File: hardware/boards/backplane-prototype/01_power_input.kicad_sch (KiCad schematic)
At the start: 13 parts, among them J5 DC IN, U4 INA237AIDGSR

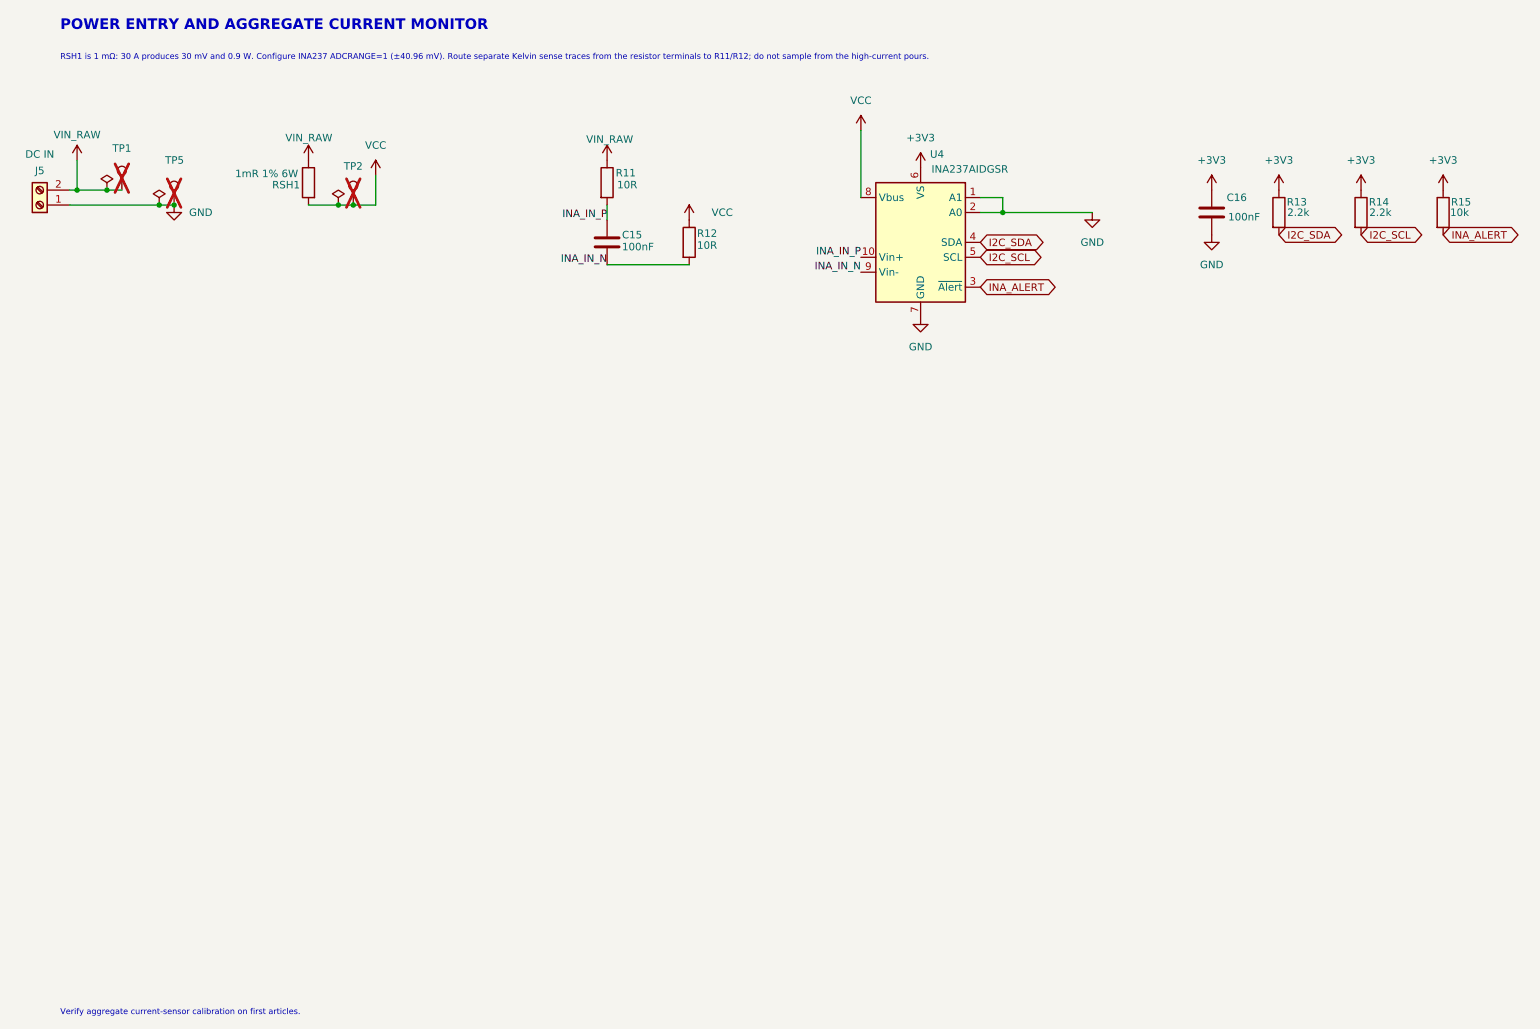
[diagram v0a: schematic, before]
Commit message: checkpoint: save schematic updates
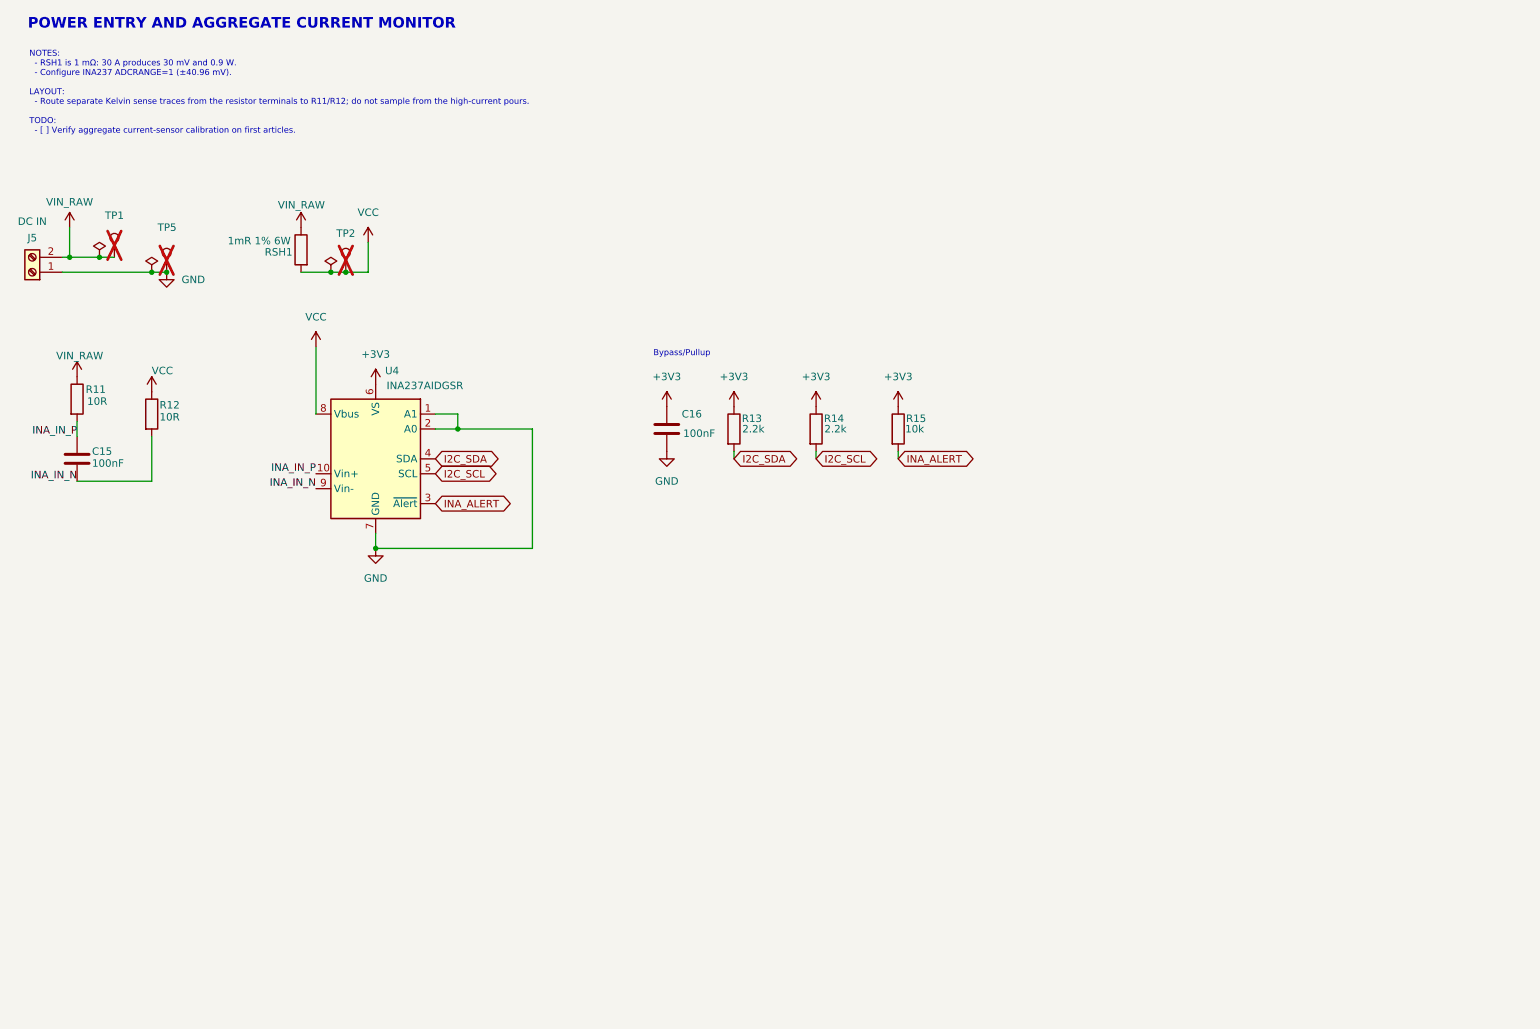
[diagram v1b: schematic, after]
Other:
- note added: "Bypass/Pullup"
- note added: "NOTES: - RSH1 is 1 mΩ: 30 A produces 30 mV and 0.9 W. - Configure INA237 ADCRANGE=1 (±40.96 mV). LAYOUT: - Route separate Kelvin sense traces from the resistor terminals to R11/R12; do not sample from the high-current pours. TODO:r - [ ] Verify aggregate current-sensor calibration on first articles."
- note removed: "RSH1 is 1 mΩ: 30 A produces 30 mV and 0.9 W. Configure INA237 ADCRANGE=1 (±40.96 mV). Route separate Kelvin sense traces from the resistor terminals to R11/R12; do not sample from the high-current pours."
- note removed: "Verify aggregate current-sensor calibration on first articles."
- moved on the sheet: C15, C16, J5, R11, R12, R13, R14, R15, RSH1, TP1, TP2, TP5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
